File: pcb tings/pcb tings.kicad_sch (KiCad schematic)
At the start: 2 parts

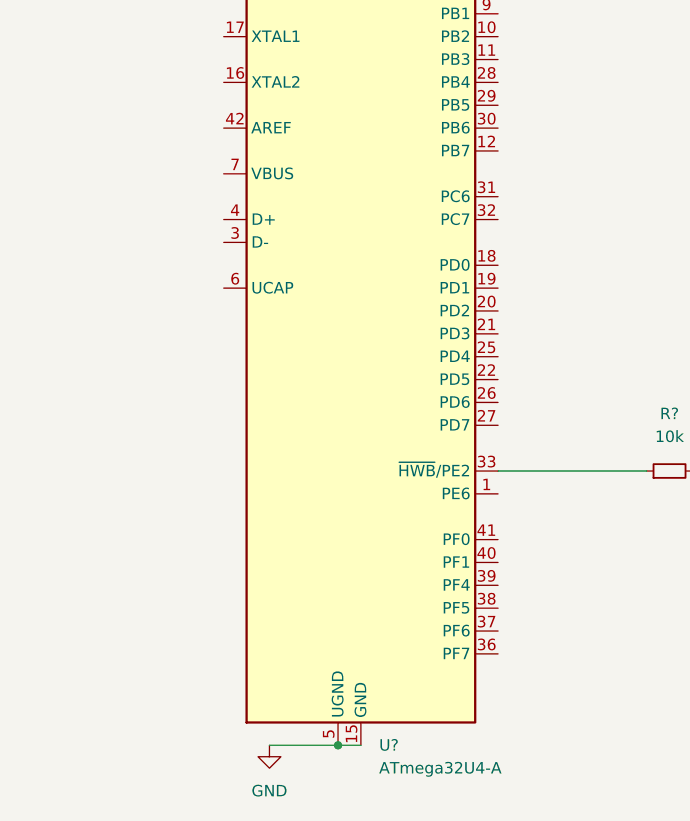
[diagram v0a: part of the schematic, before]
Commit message: Finally back to working on this
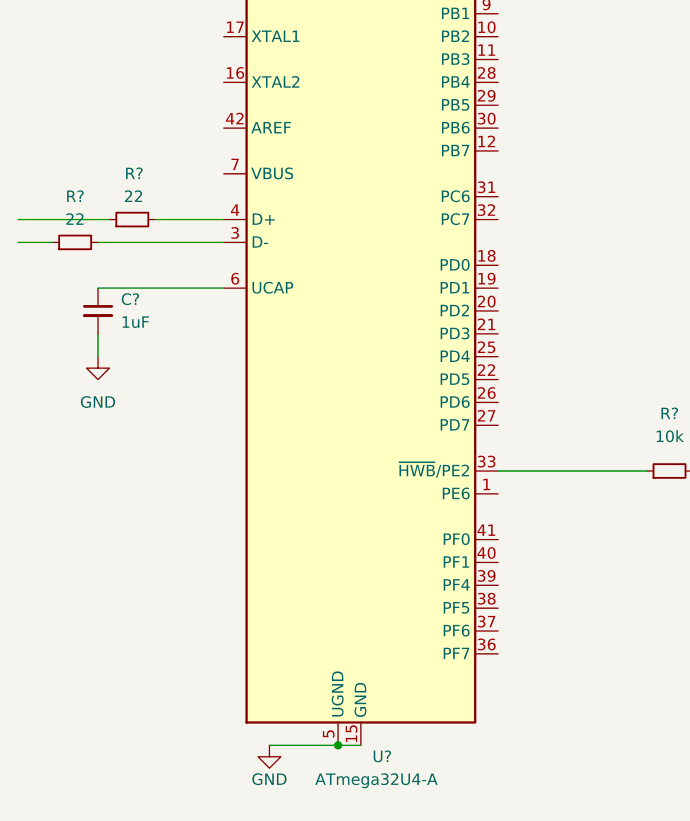
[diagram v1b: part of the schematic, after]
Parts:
- added C?: 1uF, symbol Device:C_Small
- added R? (x2): 22, symbol Device:R_Small
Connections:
- net GND: now also C?.2
- net at U?.3 (D-): now also R?.2
- net at U?.4 (D+): now also R?.2
- net at U?.6 (UCAP): now also C?.1
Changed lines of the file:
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@@
   (junction (at 55.88 50.8) (diameter 0) (color 0 0 0 0)
   )
+  (wire (pts (xy 35.56 83.82) (xy 43.18 83.82))
+    (stroke (width 0) (type default) (color 0 0 0 0))
+  )
+  (wire (pts (xy 29.21 86.36) (xy 43.18 86.36))
+    (stroke (width 0) (type default) (color 0 0 0 0))
+  )
+  (wire (pts (xy 20.32 83.82) (xy 30.48 83.82))
+    (stroke (width 0) (type default) (color 0 0 0 0))
+  )
+  (wire (pts (xy 20.32 86.36) (xy 24.13 86.36))
+    (stroke (width 0) (type default) (color 0 0 0 0))
+  )
   (wire (pts (xy 73.66 111.76) (xy 90.17 111.76))
     (stroke (width 0) (type default) (color 0 0 0 0))
@@
     (stroke (width 0) (type default) (color 0 0 0 0))
   )
+  (wire (pts (xy 29.21 91.44) (xy 43.18 91.44))
+    (stroke (width 0) (type default) (color 0 0 0 0))
+  )
   (wire (pts (xy 58.42 50.8) (xy 60.96 50.8))
+    (stroke (width 0) (type default) (color 0 0 0 0))
+  )
+  (wire (pts (xy 29.21 96.52) (xy 29.21 99.06))
     (stroke (width 0) (type default) (color 0 0 0 0))
   )
@@
     (pin "1")
   )
+  (symbol (lib_id "Device:R_Small") (at 26.67 86.36 90) (unit 1)
+    (in_bom yes) (on_board yes)
+    (property "Reference" "R?" (id 0) (at 26.67 81.28 90))
+    (property "Value" "22" (id 1) (at 26.67 83.82 90))
+    (property "Footprint" "" (id 2) (at 26.67 86.36 0)
+      (effects (font (size 1.27 1.27)) hide)
+    )
+    (property "Datasheet" "~" (id 3) (at 26.67 86.36 0)
+      (effects (font (size 1.27 1.27)) hide)
+    )
+    (pin "1")
+    (pin "2")
+  )
   (symbol (lib_id "power:+5V") (at 55.88 44.45 0) (unit 1)
     (in_bom yes) (on_board yes) (fields_autoplaced)
@@
     (pin "1")
   )
+  (symbol (lib_id "power:GND") (at 29.21 99.06 0) (unit 1)
+    (in_bom yes) (on_board yes) (fields_autoplaced)
+    (property "Reference" "#PWR?" (id 0) (at 29.21 105.41 0)
+      (effects (font (size 1.27 1.27)) hide)
+    )
+    (property "Value" "GND" (id 1) (at 29.21 104.14 0))
+    (property "Footprint" "" (id 2) (at 29.21 99.06 0)
+      (effects (font (size 1.27 1.27)) hide)
+    )
+    (property "Datasheet" "" (id 3) (at 29.21 99.06 0)
+      (effects (font (size 1.27 1.27)) hide)
+    )
+    (pin "1")
+  )
+  (symbol (lib_id "Device:R_Small") (at 33.02 83.82 90) (unit 1)
+    (in_bom yes) (on_board yes)
+    (property "Reference" "R?" (id 0) (at 34.29 78.74 90)
+      (effects (font (size 1.27 1.27)) (justify left))
+    )
+    (property "Value" "22" (id 1) (at 34.29 81.28 90)
+      (effects (font (size 1.27 1.27)) (justify left))
+    )
+    (property "Footprint" "" (id 2) (at 33.02 83.82 0)
+      (effects (font (size 1.27 1.27)) hide)
+    )
+    (property "Datasheet" "~" (id 3) (at 33.02 83.82 0)
+      (effects (font (size 1.27 1.27)) hide)
+    )
+    (pin "1")
+    (pin "2")
+  )
   (symbol (lib_id "MCU_Microchip_ATmega:ATmega32U4-A") (at 58.42 96.52 0) (unit 1)
-    (in_bom yes) (on_board yes) (fields_autoplaced)
-    (property "Reference" "U?" (id 0) (at 60.4394 142.24 0)
-      (effects (font (size 1.27 1.27)) (justify left))
-    )
-    (property "Value" "ATmega32U4-A" (id 1) (at 60.4394 144.78 0)
+    (in_bom yes) (on_board yes)
+    (property "Reference" "U?" (id 0) (at 59.69 143.51 0)
+      (effects (font (size 1.27 1.27)) (justify left))
+    )
+    (property "Value" "ATmega32U4-A" (id 1) (at 53.34 146.05 0)
       (effects (font (size 1.27 1.27)) (justify left))
     )
@@
   )
   (symbol (lib_id "power:GND") (at 48.26 142.24 0) (unit 1)
-    (in_bom yes) (on_board yes) (fields_autoplaced)
+    (in_bom yes) (on_board yes)
     (property "Reference" "#PWR?" (id 0) (at 48.26 148.59 0)
       (effects (font (size 1.27 1.27)) hide)
     )
-    (property "Value" "GND" (id 1) (at 48.26 147.32 0))
+    (property "Value" "GND" (id 1) (at 48.26 146.05 0))
     (property "Footprint" "" (id 2) (at 48.26 142.24 0)
       (effects (font (size 1.27 1.27)) hide)
@@
     (pin "2")
   )
+  (symbol (lib_id "Device:C_Small") (at 29.21 93.98 0) (unit 1)
+    (in_bom yes) (on_board yes) (fields_autoplaced)
+    (property "Reference" "C?" (id 0) (at 31.75 92.7162 0)
+      (effects (font (size 1.27 1.27)) (justify left))
+    )
+    (property "Value" "1uF" (id 1) (at 31.75 95.2562 0)
+      (effects (font (size 1.27 1.27)) (justify left))
+    )
+    (property "Footprint" "" (id 2) (at 29.21 93.98 0)
+      (effects (font (size 1.27 1.27)) hide)
+    )
+    (property "Datasheet" "~" (id 3) (at 29.21 93.98 0)
+      (effects (font (size 1.27 1.27)) hide)
+    )
+    (pin "1")
+    (pin "2")
+  )
   (sheet_instances
     (path "/" (page "1"))
@@
       (reference "#PWR?") (unit 1) (value "+5V") (footprint "")
     )
+    (path "/afa30aab-dcdf-4492-b0da-da07511df226"
+      (reference "#PWR?") (unit 1) (value "GND") (footprint "")
+    )
     (path "/b6b05379-33d6-4201-bb25-f13b46745b60"
       (reference "#PWR?") (unit 1) (value "GND") (footprint "")
     )
+    (path "/d5f3ae9d-63b3-4045-bc16-4f0d0bf26073"
+      (reference "C?") (unit 1) (value "1uF") (footprint "")
+    )
+    (path "/7c2e75b3-ed26-4254-b6d2-b338f546c2e5"
+      (reference "R?") (unit 1) (value "22") (footprint "")
+    )
+    (path "/b07e4fa3-ea3e-4f85-8ece-bb79c07ff759"
+      (reference "R?") (unit 1) (value "22") (footprint "")
+    )
     (path "/ca5557ee-df94-426c-a0ce-8db8275385ae"

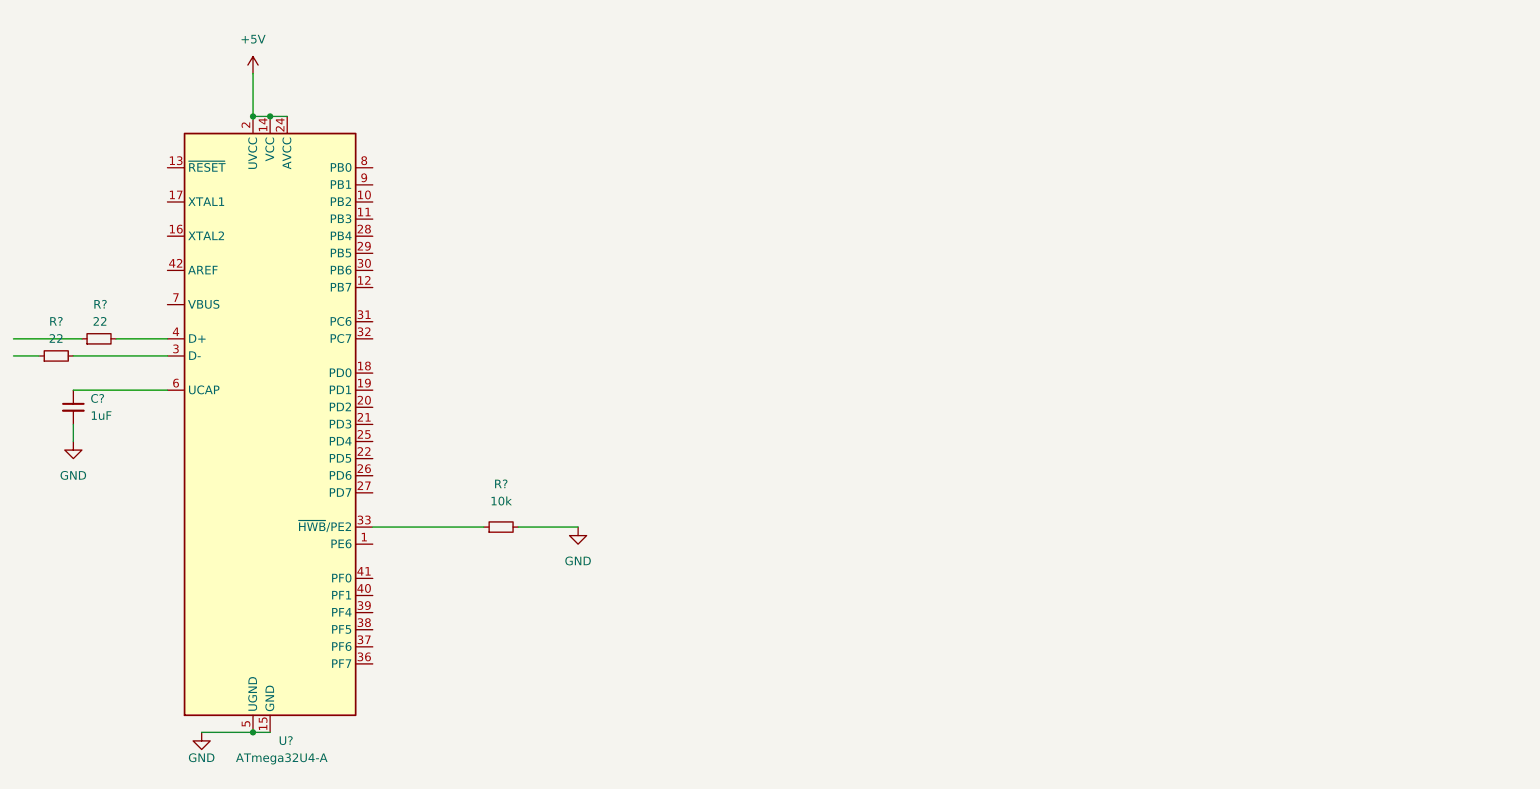
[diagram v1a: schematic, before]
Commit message: completed MCU zone
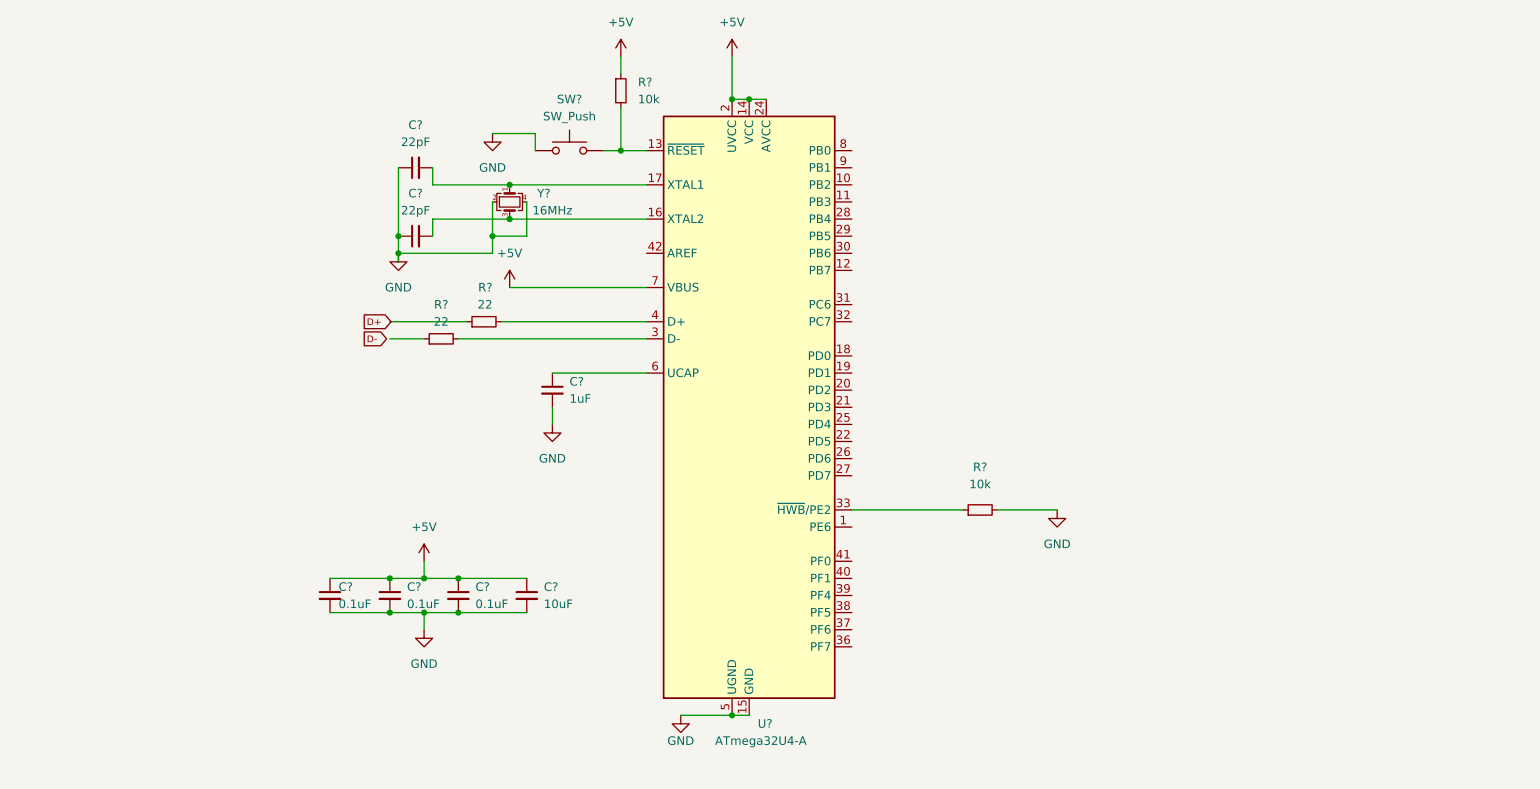
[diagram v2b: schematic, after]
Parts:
- added C? (x2): 22pF, symbol Device:C_Small
- added C? (x3): 0.1uF, symbol Device:C_Small
- added C?: 10uF, symbol Device:C_Small
- added R?: 10k, symbol Device:R_Small
- added SW?: SW_Push, symbol Switch:SW_Push
- added Y?: 16MHz, symbol Device:Crystal_GND24_Small
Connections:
- net +5V: now also U?.7 (VBUS), C?.1, C?.1, C?.1, C?.1, R?.1
- net GND: now also C?.1, C?.1, C?.2, C?.2, C?.2, C?.2, SW?.1, Y?.2, Y?.4
- net at U?.13 (~{RESET}): now also R?.2, SW?.2
- net at U?.16 (XTAL2): now also C?.2, Y?.3
- net at U?.17 (XTAL1): now also C?.2, Y?.1
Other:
- moved on the sheet: C?, R?, U?

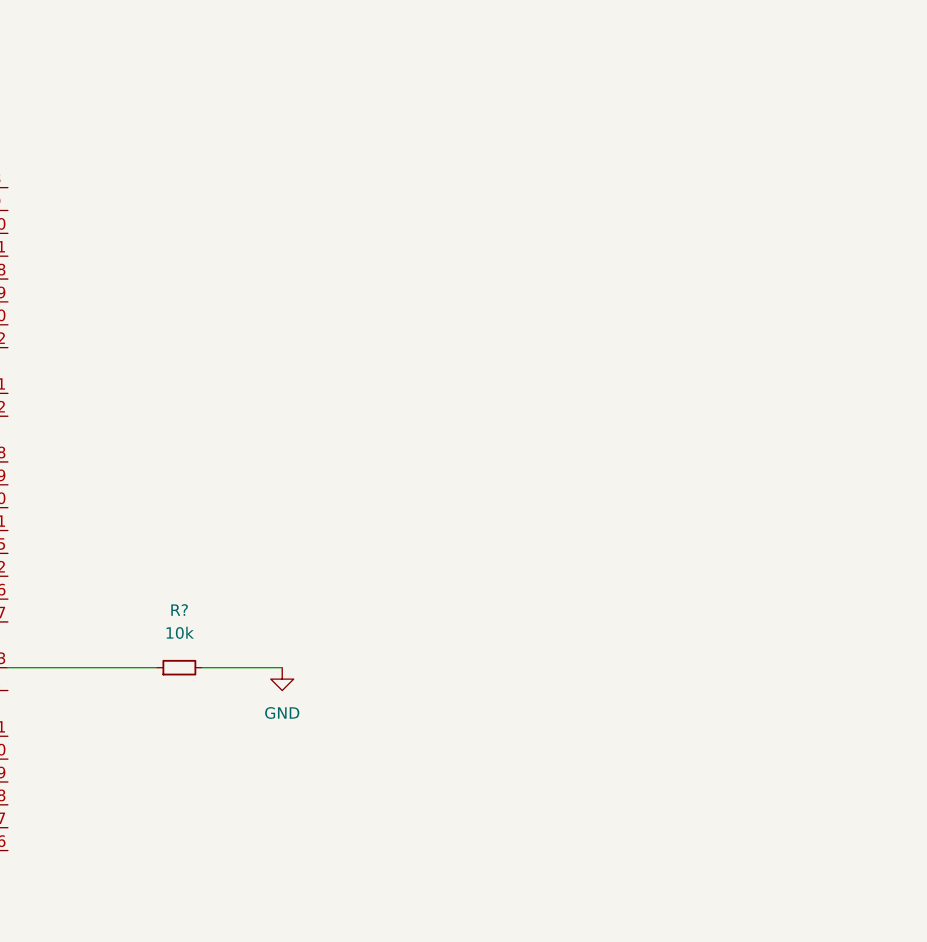
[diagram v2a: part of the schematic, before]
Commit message: power
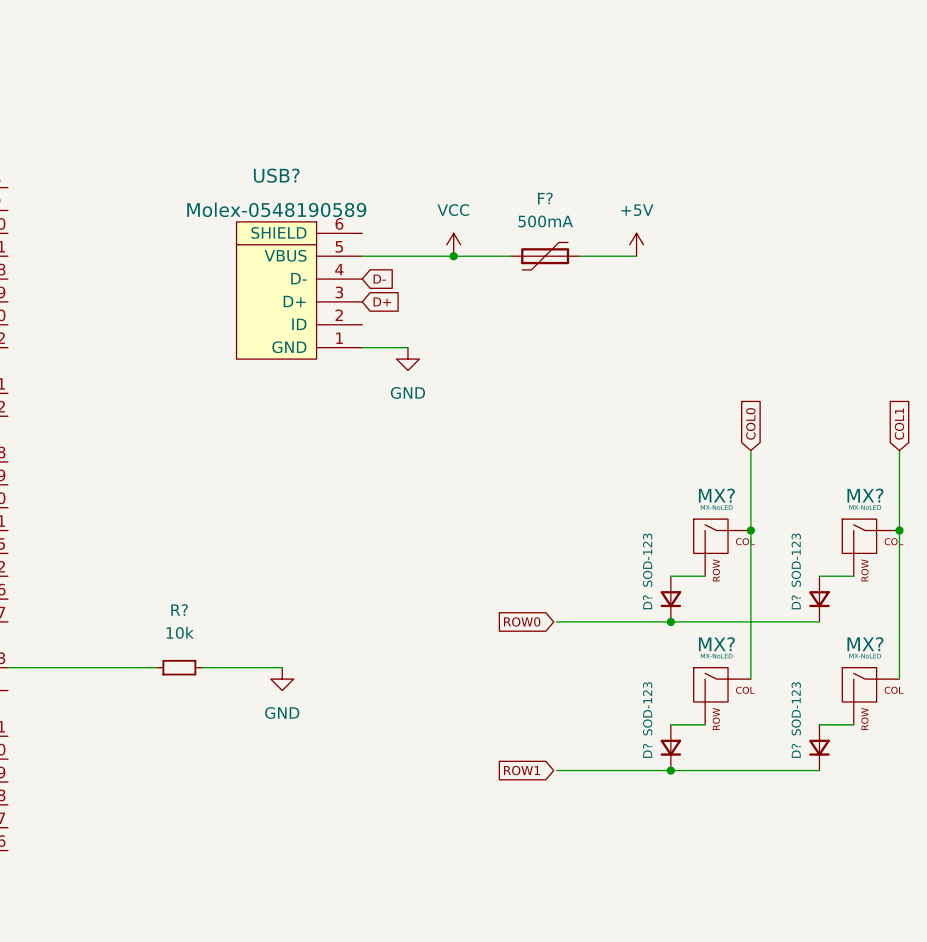
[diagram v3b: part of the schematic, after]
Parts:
- added D? (x4): SOD-123, symbol Device:D_Small
- added F?: 500mA, symbol Device:Polyfuse
- added MX? (x4): MX-NoLED, symbol MX_Alps_Hybrid:MX-NoLED
- added USB?: Molex-0548190589, symbol random-keyboard-parts:Molex-0548190589
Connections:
- net +5V: now also F?.2
- net D+: now also USB?.3 (D+)
- net D-: now also USB?.4 (D-)
- net GND: now also USB?.1 (GND)
- new net: D?.2 (A), MX?.2 (ROW) (x4)
- new net: D?.1 (K), D?.1 (K) (x2)
- new net COL0: MX?.1 (COL), MX?.1 (COL)
- new net COL1: MX?.1 (COL), MX?.1 (COL)
- new net VCC: F?.1, USB?.5 (VBUS)
